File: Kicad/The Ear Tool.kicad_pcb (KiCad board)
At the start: 2 copper layers, 57.7 x 107.7 mm, 23 parts, among them M1 MountingHole_3mm_Pad, M2 MountingHole_3mm_Pad, M3 MountingHole_3mm_Pad, M4 MountingHole_3mm_Pad, P1 AUDIO-JACK-3F07-TRS, P2 Sensor Connector, P3 9V Battery Clip, SW1 Power Switch, SW2 Full Scope Switch, SW3 Gain Switch, U1 LM386

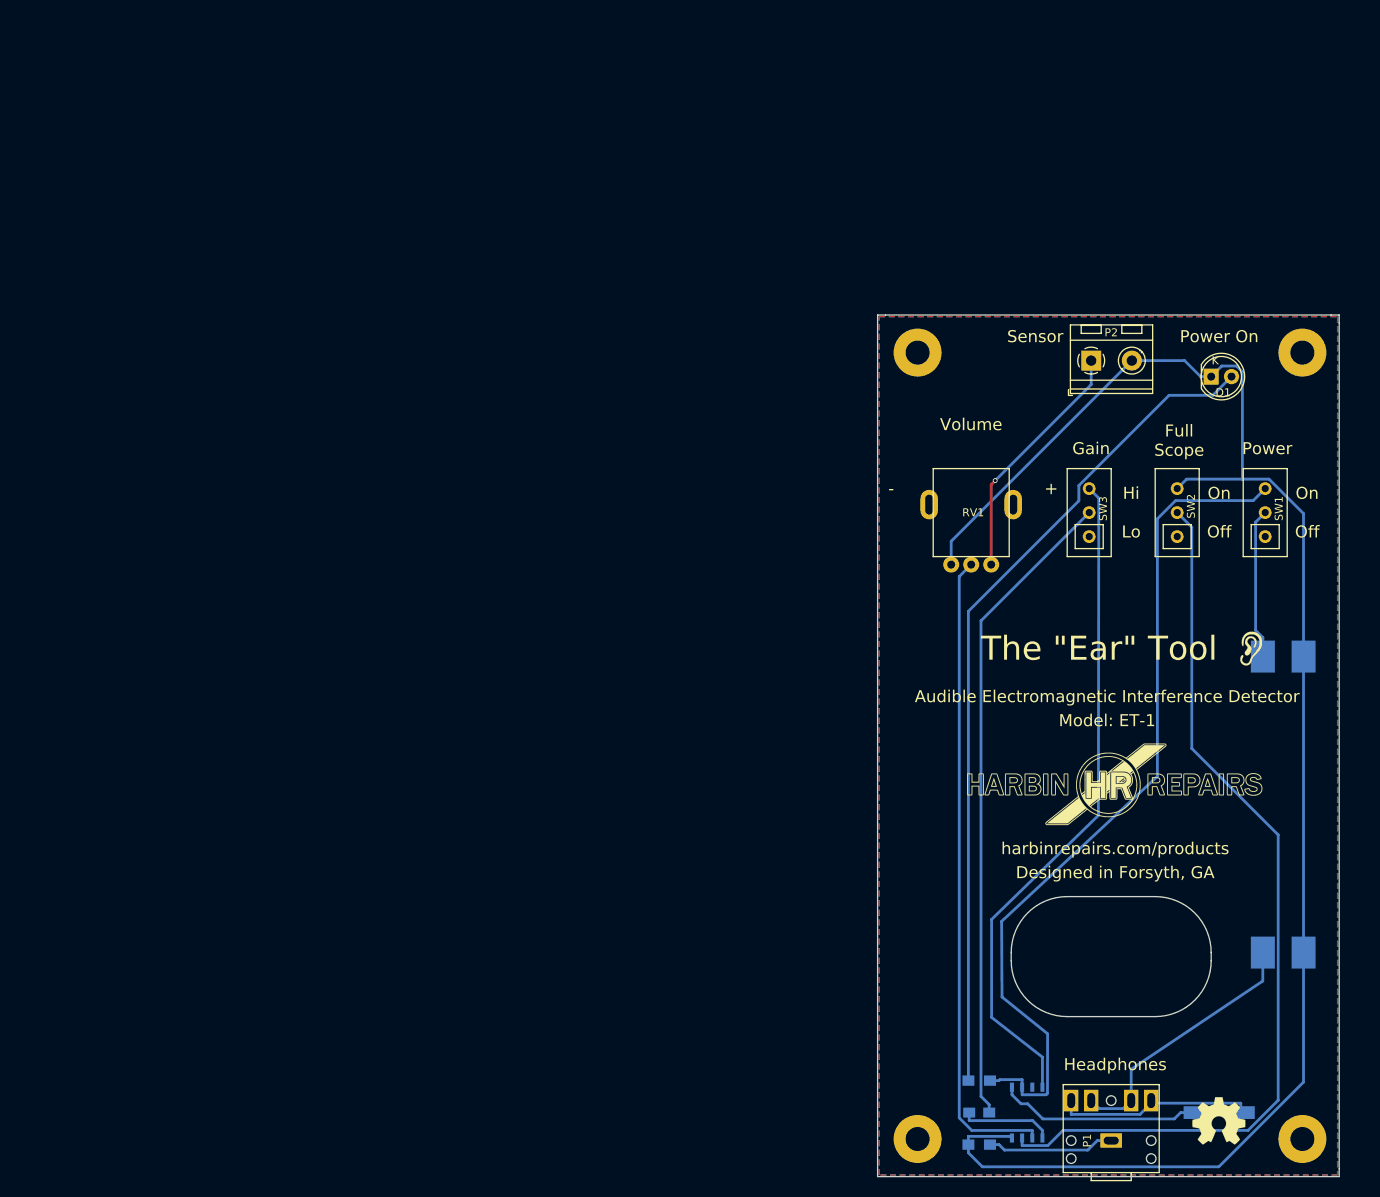
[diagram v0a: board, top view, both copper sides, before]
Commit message: Add files via upload
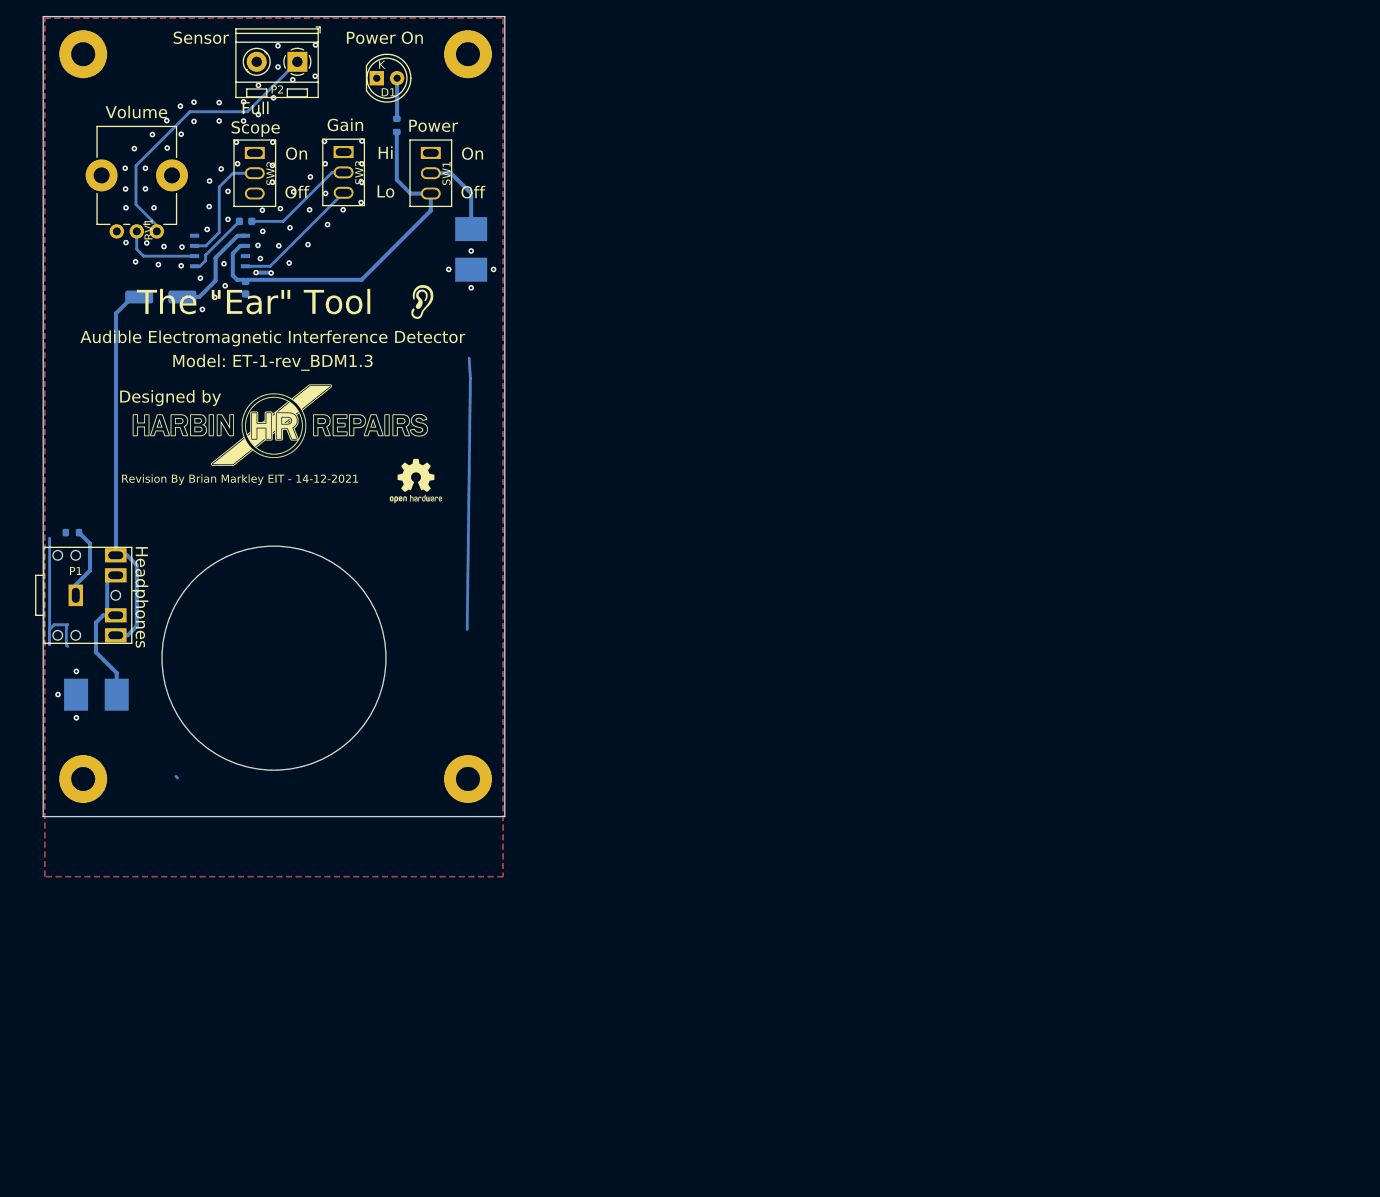
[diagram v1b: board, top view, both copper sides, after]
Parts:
- removed the REF*** at (146.9, 138.1)
- added C3: 0u1, Capacitor_SMD:C_0603_1608Metric, B.Cu at (25.3, 33.9)
- added REF***: OSHW-Logo2_7.3x6mm_SilkScreen, Symbol:OSHW-Logo2_7.3x6mm_SilkScreen, F.Cu at (46.6, 58.0)
- C1: footprint Capacitors_SMD:C_0805_HandSoldering -> Capacitor_SMD:C_0603_1608Metric
- C2: footprint Capacitors_SMD:CP_Elec_6.3x7.7 -> Capacitor_SMD:CP_Elec_6.3x7.7
- D1: footprint LEDs:LED-5MM -> LED_THT:LED_D5.0mm_Clear
- LS1, P3: footprint Oddities:NetTie-I_SMD -> SurfaceConnector:Surface Connector
- R1, R2: footprint Resistors_SMD:R_0805_HandSoldering -> Resistor_SMD:R_0603_1608Metric
- REF***: value OSHW-Symbol_6.7x6mm_SilkScreen -> OSHW-Logo2_7.3x6mm_SilkScreen; footprint Symbols:OSHW-Symbol_6.7x6mm_SilkScreen -> Symbol:OSHW-Logo2_7.3x6mm_SilkScreen
- RV1: footprint myFootprints:POT_RV09_HORIZONTAL_WHO9 -> Potentiometer_THT:Potentiometer_Bourns_PTV09A-1_Single_Vertical
- SW1, SW2, SW3: footprint myFootprints:SW_SPDT_3P_11.1mm_5.5mm -> Switch:SPDT_generic_toggle
- moved C2 167.0 mm to (14.7, 35.0), turned to 180 degrees
- moved LS1 151.8 mm to (6.65, 84.8), turned to 0 degrees
- moved U1 147.6 mm to (22.1, 29.3), turned to 90 degrees
- moved P1 144.5 mm to (5.57, 72.8), turned to 0 degrees
- moved C1 144.3 mm to (25.3, 25.6)
- moved R1 139.8 mm to (44.2, 13.6), turned to 90 degrees
- moved R2 136.7 mm to (3.65, 64.5)
- moved SW2 125.9 mm to (26.5, 19.6), turned to 270 degrees
- moved SW1 115.6 mm to (48.5, 19.6), turned to 270 degrees
- moved M3 113.6 mm to (53.1, 95.3)
- moved M4 113.6 mm to (5.00, 95.3)
- moved G1 113.6 mm to (29.7, 51.1)
- moved P3 113.5 mm to (53.5, 29.1), turned to 270 degrees
- moved G2 112.5 mm to (29.5, 51.4)
- moved G3 112.3 mm to (47.4, 35.7)
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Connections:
- R1 pad 1: Net-(D1-Pad2) -> Net-(C3-Pad2)
- R1 pad 2: Net-(R1-Pad2) -> Net-(D1-Pad2)
- RV1 pad 1: GND -> Net-(P2-Pad1)
- RV1 pad 3: Net-(P2-Pad1) -> GND
- SW1 pad 3: Net-(R1-Pad2) -> Net-(C3-Pad2)
- U1 pad 6: Net-(R1-Pad2) -> Net-(C3-Pad2)
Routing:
- net GND: track 207.5 -> 56.7 mm, vias 0 -> 79
- net Net-(R1-Pad2): track 107.3 -> 0.00 mm
- net Net-(D1-Pad2): track 104.8 -> 5.09 mm
- net Net-(SW2-Pad2): track 114.0 -> 14.6 mm
- net SENSE: track 80.5 -> 10.6 mm
- net Net-(SW3-Pad3): track 84.1 -> 16.1 mm
- net Net-(C1-Pad2): track 81.0 -> 14.0 mm
- net Net-(C3-Pad2): track 0.00 -> 46.5 mm
- net Net-(C2-Pad2): track 25.0 -> 48.0 mm
- net Net-(LS1-Pad2): track 33.1 -> 19.4 mm
- net Net-(C2-Pad1): track 25.7 -> 12.6 mm
- net +9V: track 18.9 -> 10.6 mm
- net Net-(P1-Pad1): track 15.9 -> 9.15 mm
- net Net-(P2-Pad1): track 30.7 -> 34.1 mm, vias 1 -> 0
- net Net-(C1-Pad1): track 11.6 -> 8.33 mm
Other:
- board size 57.7 x 107.7 mm -> 57.7 x 100 mm
- net class Default: via_dia 0.6 -> 0.7; via_drill 0.4 -> 0.3
- rule pad_to_mask_clearance: 0.2 -> 0
- board text added: "Model: ET-1-rev_BDM1.3"
- board text added: "Revision By Brian Markley EIT - 14-12-2021"
- board text removed: "+"
- board text removed: "-"
- board text removed: "2019"
- board text removed: "Designed in Forsyth, GA"
- board text removed: "ET-1 Revision 1.3"
- board text removed: "Model: ET-1"
- board text removed: "harbinrepairs.com/products"
